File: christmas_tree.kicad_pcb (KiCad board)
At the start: 2 copper layers, 29 parts, among them J1 Conn_01x28_Female, J10 Conn_01x28_Female, J11 Conn_01x03_Female, J2 Conn_01x16_Female, J3 Conn_01x12_Female, J4 Conn_01x16_Female, J5 Conn_01x12_Female, J6 Conn_01x12_Female, J7 Conn_01x16_Female, J8 Conn_01x12_Female, J9 Conn_01x16_Female, U1 TLC5940PWP, U2 TLC5940PWP, U3 ATTINY13-20SSU, U4 TLC5940PWP, U5 TLC5940PWP, U6 TLC5940PWP, U7 TLC5940PWP, U8 TLC5940PWP, U9 TLC5940PWP

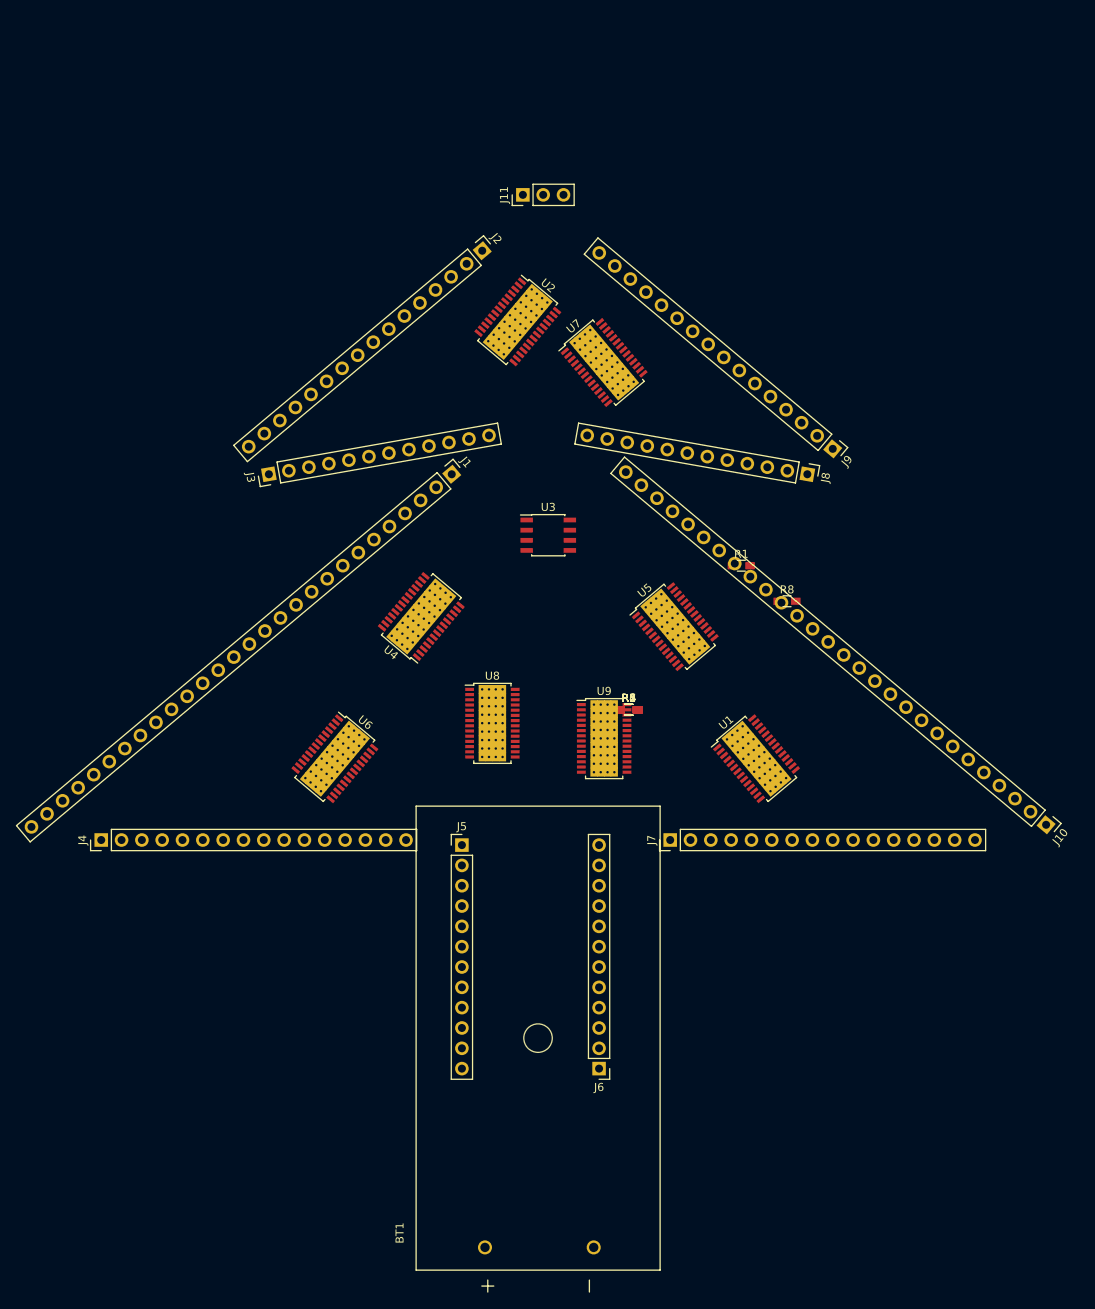
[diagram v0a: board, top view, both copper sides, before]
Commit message: Christmas tree edge cut
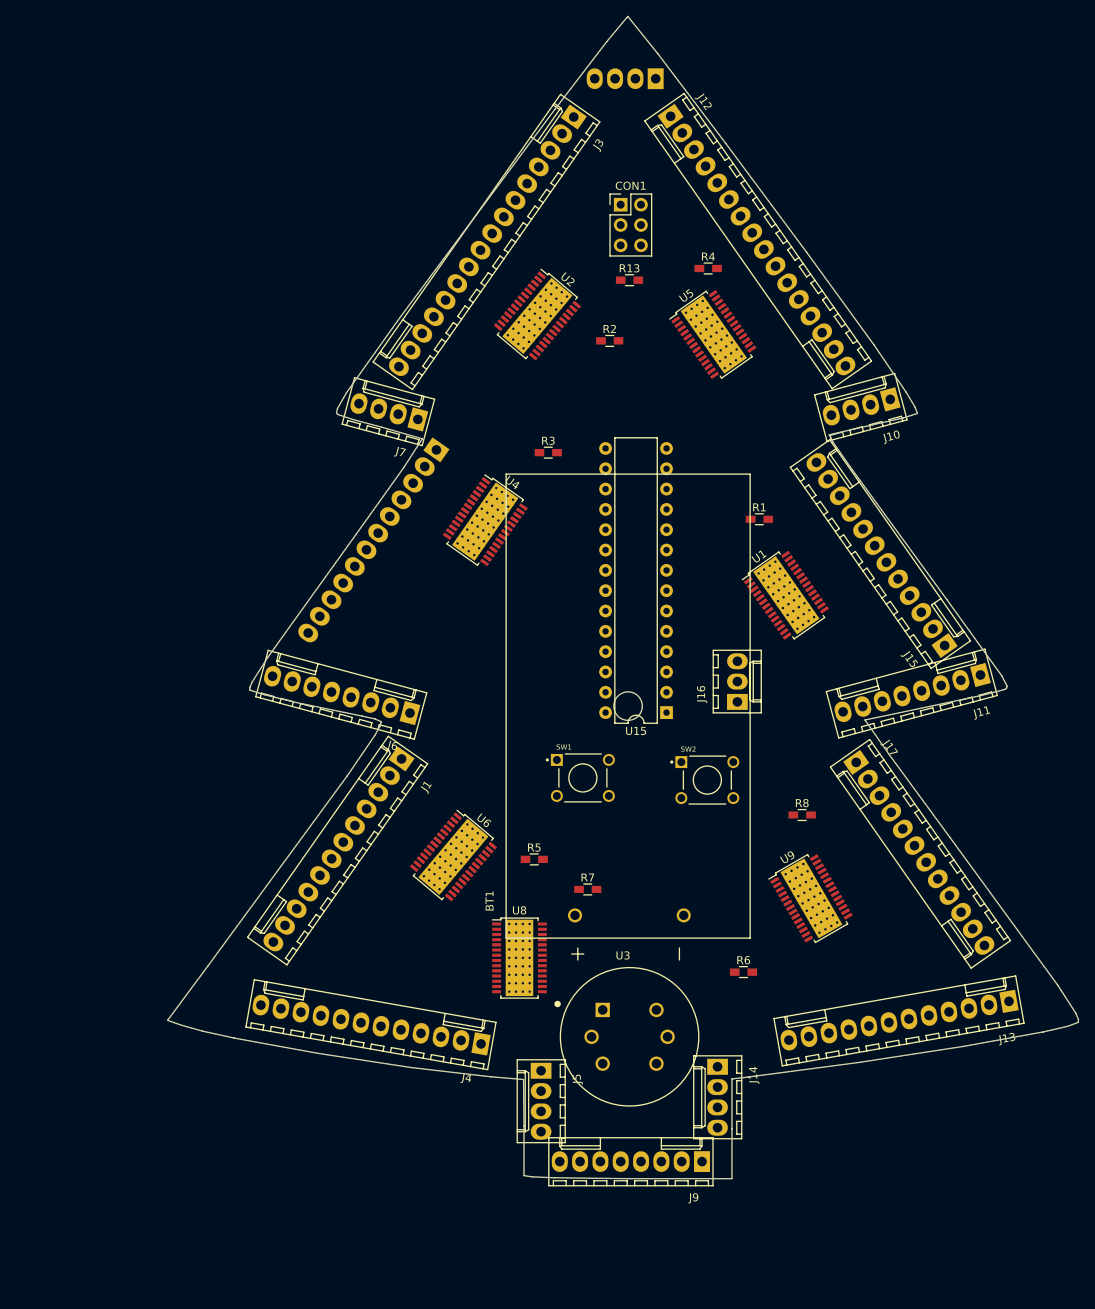
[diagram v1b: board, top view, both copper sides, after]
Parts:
- removed U7: TLC5940PWP, Housings_SSOP:HTSSOP-28_4.4x9.7mm_Pitch0.65mm_ThermalPad
- added CON1: AVR-ISP-6, Pin_Headers:Pin_Header_Straight_2x03_Pitch2.54mm, F.Cu at (147.5, 41.9)
- added J12: Conn_01x16_Female, Connectors_Molex:Molex_KK-6410-16_16x2.54mm_Straight, F.Cu at (153.7, 30.8)
- added J13: Conn_01x12_Female, Connectors_Molex:Molex_KK-6410-12_12x2.54mm_Straight, F.Cu at (196.0, 141.5)
- added J14: Conn_01x04_Female, Connectors_Molex:Molex_KK-6410-04_04x2.54mm_Straight, F.Cu at (159.6, 149.6)
- added J15: Conn_01x12_Female, Connectors_Molex:Molex_KK-6410-12_12x2.54mm_Straight, F.Cu at (188.0, 97.0)
- added J16: Conn_01x03_Male, Connectors_Molex:Molex_KK-6410-03_03x2.54mm_Straight, F.Cu at (162.1, 104.0)
- added J17: Conn_01x12_Female, Connectors_Molex:Molex_KK-6410-12_12x2.54mm_Straight, F.Cu at (176.9, 111.6)
- added R13: 10k, Resistors_SMD:R_0603_HandSoldering, F.Cu at (148.6, 51.3)
- added SW1: 1825910-6, snapeda_pushbutton:SW_1825910-6-4, F.Cu at (142.8, 113.5)
- added SW2: 1825910-6, snapeda_pushbutton:SW_1825910-6-4, F.Cu at (158.3, 113.8)
- added U15: ATMEGA48-20PU, Housings_DIP:DIP-28_W7.62mm, F.Cu at (153.2, 105.4)
- J1: value Conn_01x28_Female -> Conn_01x12_Female; footprint Pin_Headers:Pin_Header_Straight_1x28_Pitch2.54mm -> Connectors_Molex:Molex_KK-6410-12_12x2.54mm_Straight
- J10: value Conn_01x28_Female -> Conn_01x04_Female; footprint Pin_Headers:Pin_Header_Straight_1x28_Pitch2.54mm -> Connectors_Molex:Molex_KK-6410-04_04x2.54mm_Straight
- J11: value Conn_01x03_Female -> Conn_01x08_Female; footprint Pin_Headers:Pin_Header_Straight_1x03_Pitch2.54mm -> Connectors_Molex:Molex_KK-6410-08_08x2.54mm_Straight
- J2, J4: value Conn_01x16_Female -> Conn_01x12_Female; footprint Pin_Headers:Pin_Header_Straight_1x16_Pitch2.54mm -> Connectors_Molex:Molex_KK-6410-12_12x2.54mm_Straight
- J3: value Conn_01x12_Female -> Conn_01x16_Female; footprint Pin_Headers:Pin_Header_Straight_1x12_Pitch2.54mm -> Connectors_Molex:Molex_KK-6410-16_16x2.54mm_Straight
- J5, J8: value Conn_01x12_Female -> Conn_01x04_Female; footprint Pin_Headers:Pin_Header_Straight_1x12_Pitch2.54mm -> Connectors_Molex:Molex_KK-6410-04_04x2.54mm_Straight
- J6: value Conn_01x12_Female -> Conn_01x08_Female; footprint Pin_Headers:Pin_Header_Straight_1x12_Pitch2.54mm -> Connectors_Molex:Molex_KK-6410-08_08x2.54mm_Straight
- J7: value Conn_01x16_Female -> Conn_01x04_Female; footprint Pin_Headers:Pin_Header_Straight_1x16_Pitch2.54mm -> Connectors_Molex:Molex_KK-6410-04_04x2.54mm_Straight
- J9: value Conn_01x16_Female -> Conn_01x08_Female; footprint Pin_Headers:Pin_Header_Straight_1x16_Pitch2.54mm -> Connectors_Molex:Molex_KK-6410-08_08x2.54mm_Straight
- R6: value 1.5 -> 10k
- U3: value ATTINY13-20SSU -> SEN-08880; footprint Housings_SOIC:SOIC-8_3.9x4.9mm_Pitch1.27mm -> SEN-08880:XDCR_SEN-08880
- moved J9 90.6 mm to (157.6, 161.5), turned to 180 degrees
- moved J11 82.9 mm to (192.5, 100.7), turned to 195 degrees
- moved U3 63.5 mm to (148.6, 145.9)
- moved J7 61.3 mm to (122.1, 68.7), turned to 165 degrees
- moved J3 58.7 mm to (141.6, 30.9), turned to 235 degrees
- moved J10 56.6 mm to (181.2, 66.2), turned to 195 degrees
- moved R4 56.0 mm to (158.4, 49.8)
- moved J4 53.9 mm to (130.0, 146.8), turned to 170 degrees
- moved J8 53.0 mm to (151.9, 26.1), turned to 180 degrees
- moved J6 50.3 mm to (121.1, 105.4), turned to 165 degrees
- moved R2 46.2 mm to (146.1, 58.9)
- moved BT1 43.0 mm to (148.4, 104.5)
- moved U5 36.8 mm to (159.1, 58.1), turned to 35 degrees
- moved J1 36.1 mm to (120.1, 111.2), turned to 235 degrees
- moved R6 35.8 mm to (162.8, 137.8)
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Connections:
- BT1 pad +: VCC -> Net-(BT1-Pad+)
- J1 pad 1: /O15 -> /O115
- J1 pad 11: /O112 -> /O26
- J1 pad 12: /O113 -> /O27
- J1 pad 3: /O16 -> /O20
- J1 pad 4: /O17 -> /O21
- J1 pad 5: /O18 -> /O22
- J1 pad 7: /O19 -> /O23
- J1 pad 8: /O110 -> /O24
- J1 pad 9: /O111 -> /O25
- J10 pad 1: /O54 -> /O60
- J10 pad 2: GND -> /O515
- J10 pad 3: /O55 -> GND
- J10 pad 4: /O56 -> /O514
- J11 pad 1: /O715 -> /O54
- J11 pad 2: GND -> /O53
- J11 pad 3: /O714 -> GND
- J2 pad 1: /O00 -> /O10
- J2 pad 11: /O07 -> /O17
- J2 pad 12: /O08 -> /O18
- J2 pad 3: /O01 -> /O11
- J2 pad 4: /O02 -> /O12
- J2 pad 5: /O03 -> /O13
- J2 pad 7: /O04 -> /O14
- J2 pad 8: /O05 -> /O15
- J2 pad 9: /O06 -> /O16
- J3 pad 1: /O012 -> /O00
- J3 pad 11: /O13 -> /O07
- J3 pad 12: /O14 -> /O08
- J3 pad 3: /O013 -> /O01
- J3 pad 4: /O014 -> /O02
- J3 pad 5: /O015 -> /O03
- J3 pad 7: /O10 -> /O04
- J3 pad 8: /O11 -> /O05
- J3 pad 9: /O12 -> /O06
- J4 pad 1: /O210 -> /O30
- J4 pad 10: GND -> /O29
- J4 pad 11: /O31 -> GND
- J4 pad 12: /O32 -> /O28
- J4 pad 2: GND -> /O215
- J4 pad 3: /O211 -> GND
- J4 pad 4: /O212 -> /O214
- J4 pad 6: GND -> /O212
- J4 pad 7: /O214 -> GND
- J4 pad 8: /O215 -> /O211
- J4 pad 9: /O30 -> /O210
- J5 pad 1: /O36 -> /O31
- J5 pad 3: /O37 -> /O32
- J5 pad 4: /O38 -> /O33
- J6 pad 1: /O315 -> /O114
- J6 pad 2: GND -> /O113
- J6 pad 3: /O40 -> GND
- J6 pad 4: /O41 -> /O112
- J6 pad 5: /O42 -> /O111
- J6 pad 6: GND -> /O110
- J6 pad 7: /O43 -> GND
- J6 pad 8: /O44 -> /O19
- J7 pad 1: /O48 -> /O015
- J7 pad 2: GND -> /O014
- J7 pad 3: /O49 -> GND
- J7 pad 4: /O410 -> /O013
- J8 pad 1: /O69 -> /O613
- J8 pad 3: /O610 -> /O614
- J8 pad 4: /O611 -> /O615
- J9 pad 1: /O72 -> /O39
- J9 pad 2: GND -> /O38
- J9 pad 3: /O73 -> GND
- J9 pad 4: /O74 -> /O37
- J9 pad 5: /O75 -> /O36
- J9 pad 6: GND -> /O35
- J9 pad 7: /O76 -> GND
- J9 pad 8: /O77 -> /O34
- R6 pad 1: Net-(R6-Pad1) -> GND
- R6 pad 2: GND -> Net-(R6-Pad2)
- U2 pad 18: /O011 -> Net-(U2-Pad18)
- U3 pad 1: /VPRG -> VCC
- U3 pad 2: /XLAT -> VCC
- U3 pad 3: /BLANK -> VCC
- U3 pad 4: GND -> /MQ3_A
- U3 pad 5: /MOSI -> Net-(R6-Pad2)
- U3 pad 6: /GCLK -> /MQ3_A
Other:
- board outline added: 113.9 x 145.3 mm
